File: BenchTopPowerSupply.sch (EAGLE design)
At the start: 129 parts, among them U10 E2A-T220-25E, U7 STM32F103C8T6, U8 E2A-T220-25E, U9 E2A-T220-25E, X1 5566-24, Y1 8MHZ

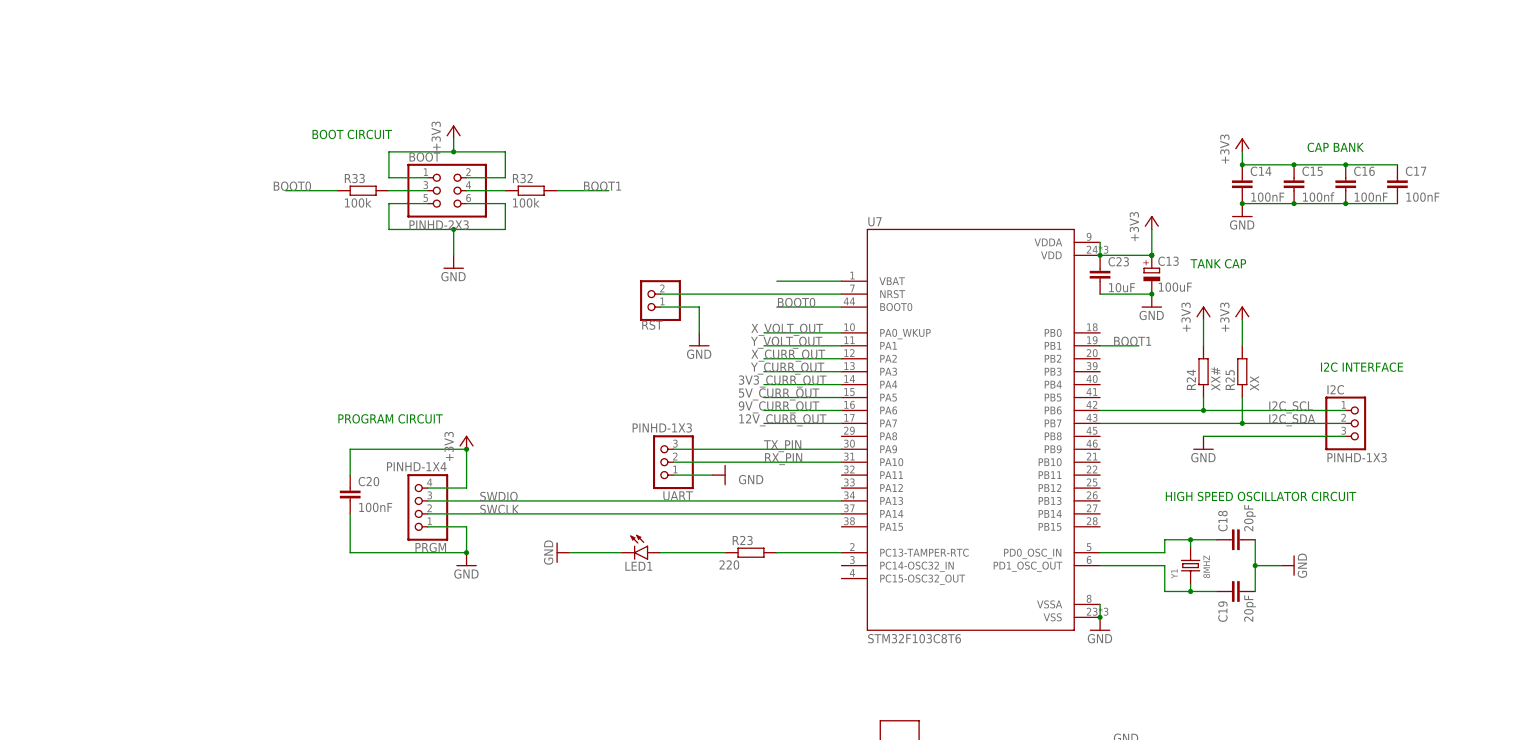
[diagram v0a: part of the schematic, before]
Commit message: Fixing schematic issues
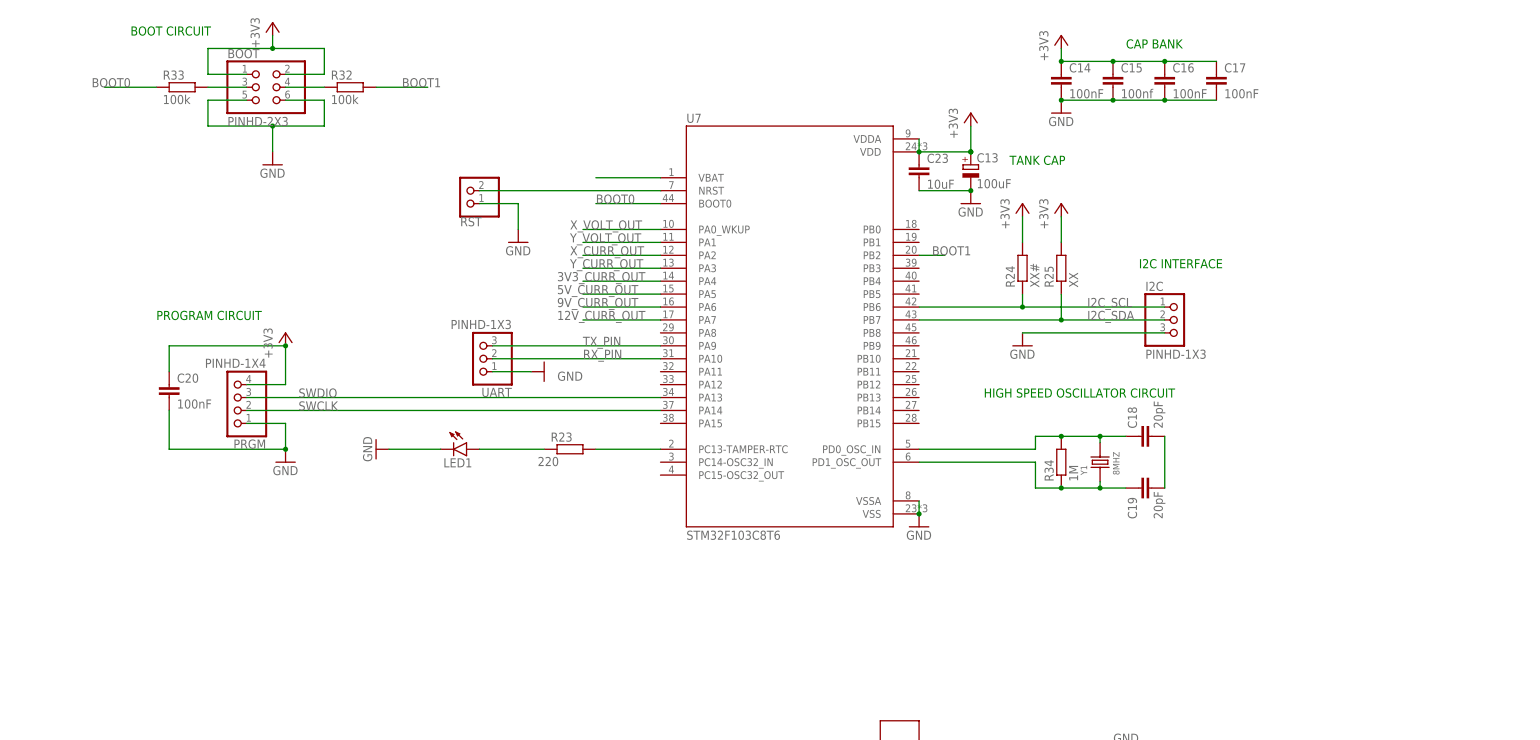
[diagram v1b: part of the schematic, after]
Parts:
- added R34: 1M, rcl:R-EU_R1206
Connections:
- new net N$10: C18.2, C19.2
- net BOOT1: now also U7.PB2; no longer U7.PB1
- net GND: no longer C18.2, C19.2
- net N$3: now also R34.2
- net N$5: now also R34.1
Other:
- moved on the sheet: BOOT, C13, C14, C15, C16, C17, C18, C19, C20, C23, I2C, LED1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
